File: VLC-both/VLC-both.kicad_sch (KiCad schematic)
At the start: 2 parts, among them J1 40HAT, J3 40HAT

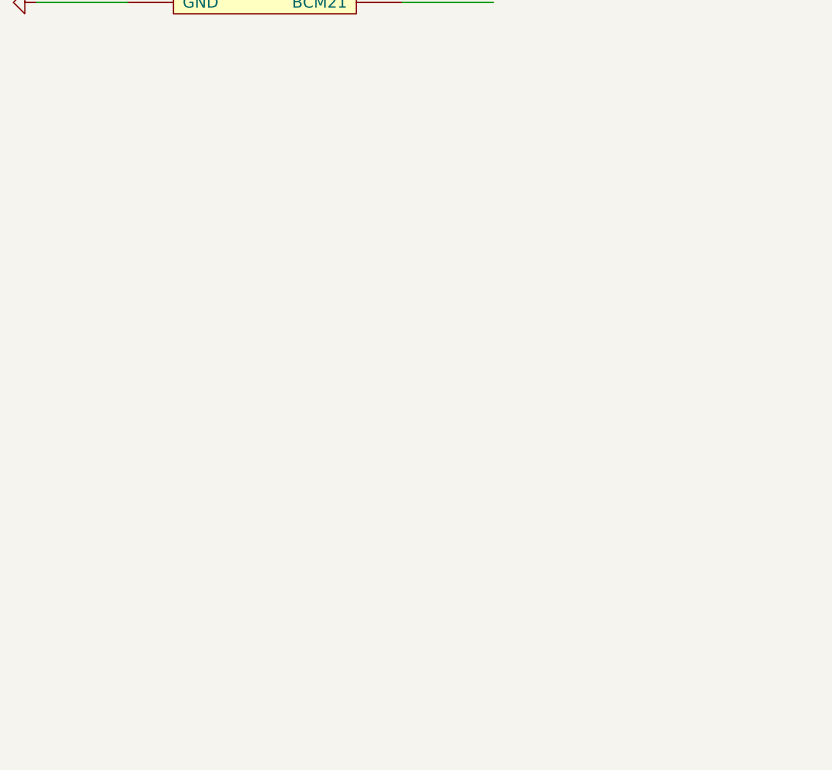
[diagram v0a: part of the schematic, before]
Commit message: h
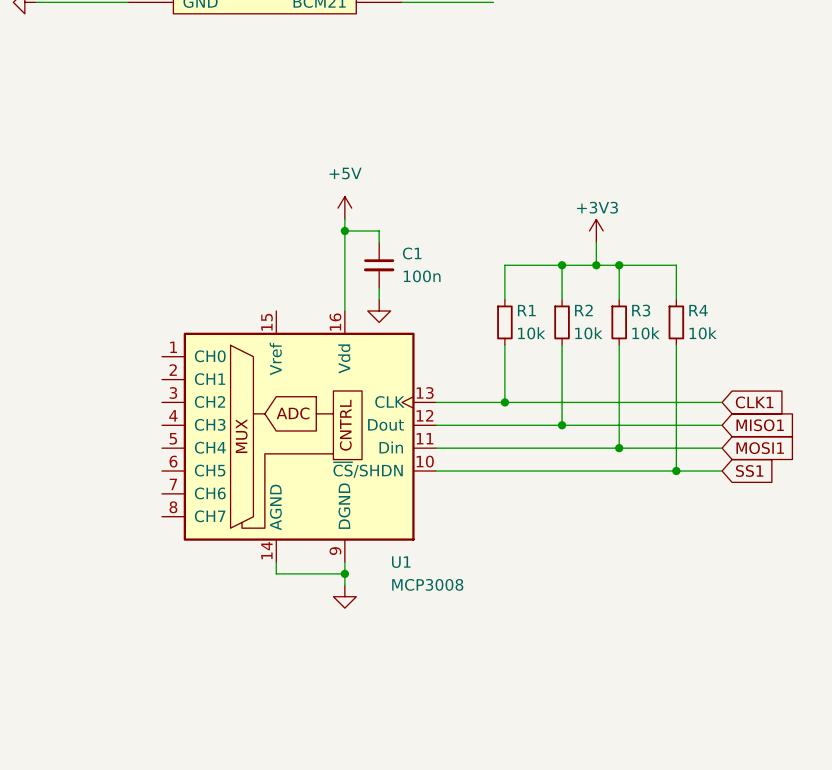
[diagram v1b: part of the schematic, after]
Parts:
- added C1: 100n, Capacitor_SMD:C_0805_2012Metric, symbol Device:C_Small
- added R1, R2, R3, R4: 10k, Resistor_SMD:R_0805_2012Metric, symbol Device:R_Small
- added U1: MCP3008, Package_SO:SOIC-16_3.9x9.9mm_P1.27mm, symbol Analog_ADC:MCP3008
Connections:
- net +3V3: now also R1.1, R2.1, R3.1, R4.1
- net +5V: now also C1.1, U1.16 (Vdd)
- net GND: now also C1.2, U1.14 (AGND), U1.9 (DGND)
- new net CLK1: R1.2, U1.13 (CLK)
- new net MISO1: R2.2, U1.12 (Dout)
- new net MOSI1: R3.2, U1.11 (Din)
- new net SS1: R4.2, U1.10 (~{CS}/SHDN)
